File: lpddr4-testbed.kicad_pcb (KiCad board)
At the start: 6 copper layers, 69.6 x 30 mm, 68 parts, among them IC1 PCA6408APW, IC2 AT24CS01, J1 ddr4-sodimm-edge-connector, U1 MT53E1G32D2NP-046, U2 TPS613221ADBVT

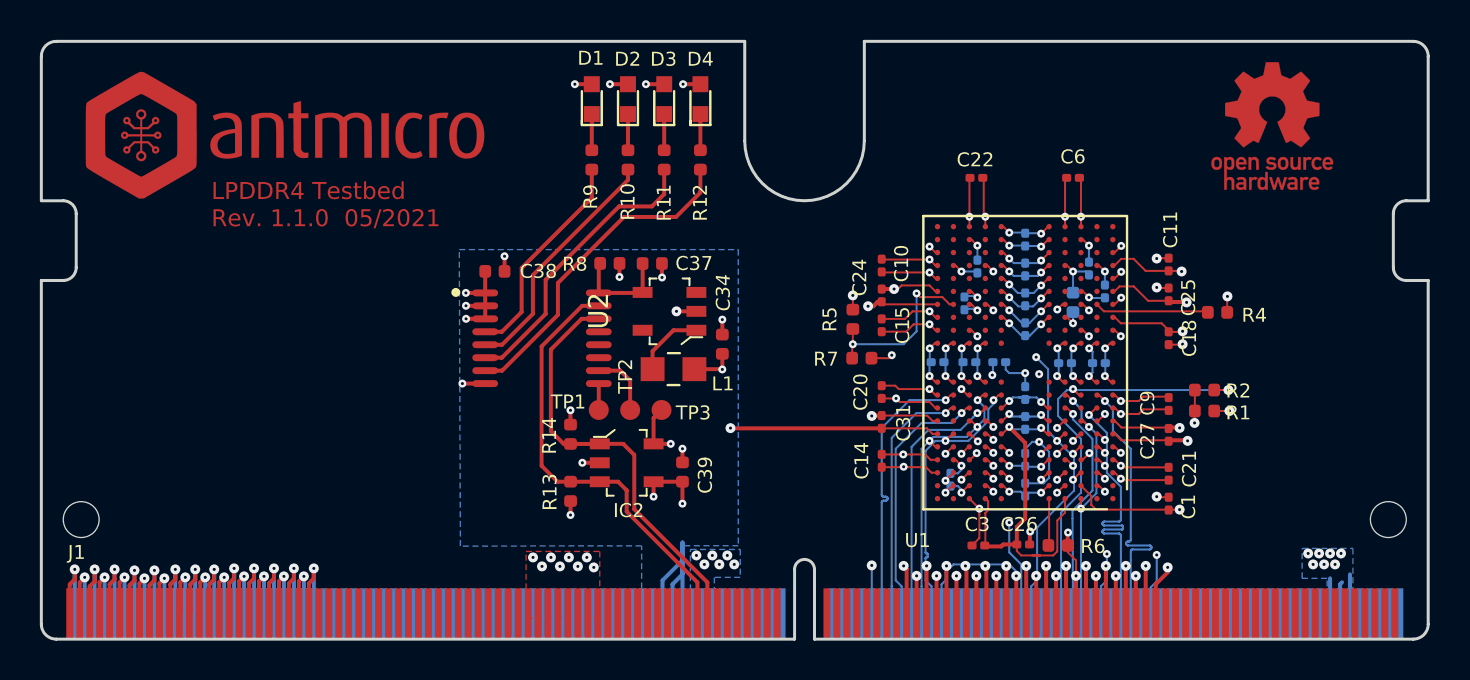
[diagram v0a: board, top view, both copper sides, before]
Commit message: Clean DRC
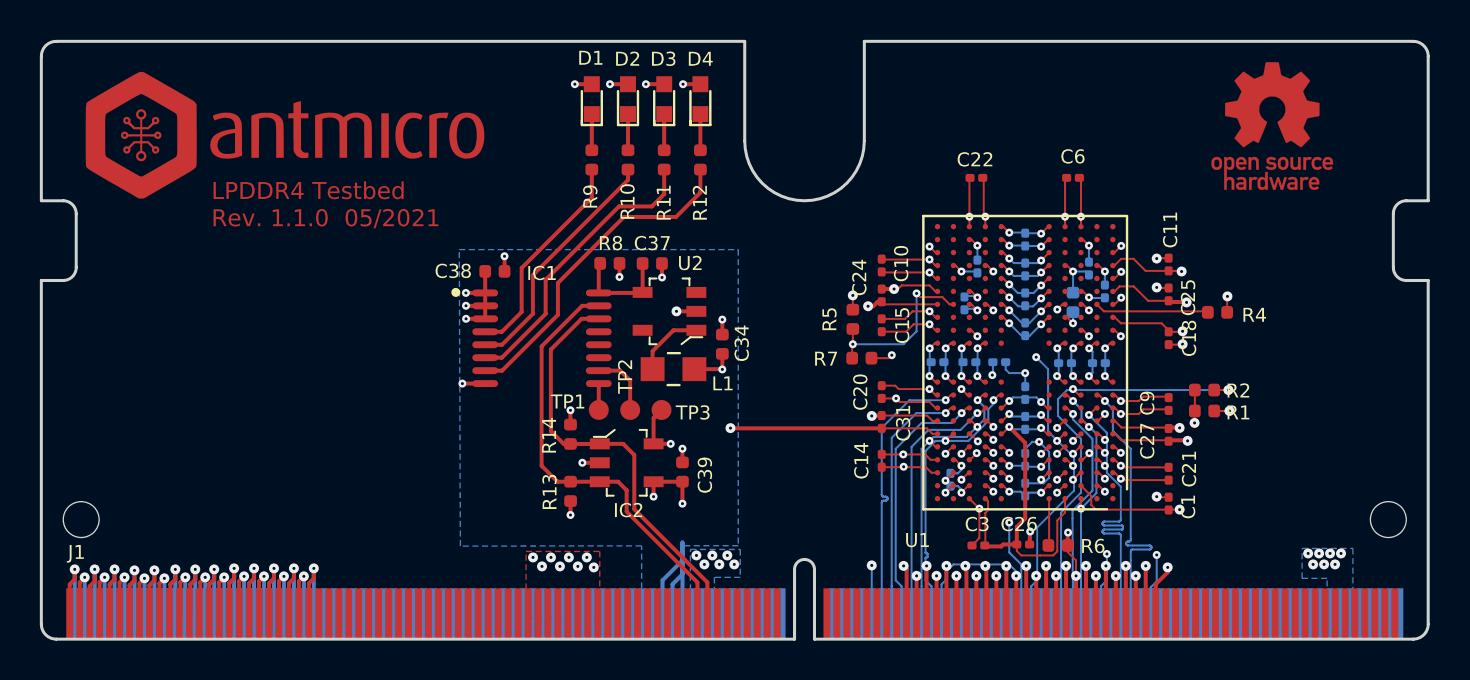
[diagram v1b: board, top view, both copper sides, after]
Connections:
- IC1 pad 11: Net-(IC1-Pad11) -> unconnected-(IC1-Pad11)
- IC1 pad 12: Net-(IC1-Pad12) -> unconnected-(IC1-Pad12)
- IC1 pad 13: Net-(IC1-Pad13) -> unconnected-(IC1-Pad13)
- J1 pad 100: Net-(J1-Pad100) -> unconnected-(J1-Pad100)
- J1 pad 102: Net-(J1-Pad102) -> unconnected-(J1-Pad102)
- J1 pad 104: Net-(J1-Pad104) -> unconnected-(J1-Pad104)
- J1 pad 106: Net-(J1-Pad106) -> unconnected-(J1-Pad106)
- J1 pad 108: Net-(J1-Pad108) -> unconnected-(J1-Pad108)
- J1 pad 109: Net-(J1-Pad109) -> unconnected-(J1-Pad109)
- J1 pad 110: Net-(J1-Pad110) -> unconnected-(J1-Pad110)
- J1 pad 111: Net-(J1-Pad111) -> unconnected-(J1-Pad111)
- J1 pad 112: Net-(J1-Pad112) -> unconnected-(J1-Pad112)
- J1 pad 113: Net-(J1-Pad113) -> unconnected-(J1-Pad113)
- J1 pad 114: Net-(J1-Pad114) -> unconnected-(J1-Pad114)
- J1 pad 115: Net-(J1-Pad115) -> unconnected-(J1-Pad115)
- J1 pad 117: Net-(J1-Pad117) -> unconnected-(J1-Pad117)
- J1 pad 119: Net-(J1-Pad119) -> unconnected-(J1-Pad119)
- J1 pad 121: Net-(J1-Pad121) -> unconnected-(J1-Pad121)
- J1 pad 123: Net-(J1-Pad123) -> unconnected-(J1-Pad123)
- J1 pad 125: Net-(J1-Pad125) -> unconnected-(J1-Pad125)
- J1 pad 131: Net-(J1-Pad131) -> unconnected-(J1-Pad131)
- J1 pad 132: Net-(J1-Pad132) -> unconnected-(J1-Pad132)
- J1 pad 133: Net-(J1-Pad133) -> unconnected-(J1-Pad133)
- J1 pad 134: Net-(J1-Pad134) -> unconnected-(J1-Pad134)
- J1 pad 135: Net-(J1-Pad135) -> unconnected-(J1-Pad135)
- J1 pad 136: Net-(J1-Pad136) -> unconnected-(J1-Pad136)
- J1 pad 137: Net-(J1-Pad137) -> unconnected-(J1-Pad137)
- J1 pad 138: Net-(J1-Pad138) -> unconnected-(J1-Pad138)
- J1 pad 139: Net-(J1-Pad139) -> unconnected-(J1-Pad139)
- J1 pad 140: Net-(J1-Pad140) -> unconnected-(J1-Pad140)
- J1 pad 141: Net-(J1-Pad141) -> unconnected-(J1-Pad141)
- J1 pad 142: Net-(J1-Pad142) -> unconnected-(J1-Pad142)
- J1 pad 143: Net-(J1-Pad143) -> unconnected-(J1-Pad143)
- J1 pad 144: Net-(J1-Pad144) -> unconnected-(J1-Pad144)
- J1 pad 145: Net-(J1-Pad145) -> unconnected-(J1-Pad145)
- J1 pad 146: Net-(J1-Pad146) -> unconnected-(J1-Pad146)
- J1 pad 147: Net-(J1-Pad147) -> unconnected-(J1-Pad147)
- J1 pad 148: Net-(J1-Pad148) -> unconnected-(J1-Pad148)
- J1 pad 149: Net-(J1-Pad149) -> unconnected-(J1-Pad149)
- J1 pad 150: Net-(J1-Pad150) -> unconnected-(J1-Pad150)
- J1 pad 151: Net-(J1-Pad151) -> unconnected-(J1-Pad151)
- J1 pad 152: Net-(J1-Pad152) -> unconnected-(J1-Pad152)
- J1 pad 153: Net-(J1-Pad153) -> unconnected-(J1-Pad153)
- J1 pad 155: Net-(J1-Pad155) -> unconnected-(J1-Pad155)
- J1 pad 157: Net-(J1-Pad157) -> unconnected-(J1-Pad157)
- J1 pad 159: Net-(J1-Pad159) -> unconnected-(J1-Pad159)
- J1 pad 170: Net-(J1-Pad170) -> unconnected-(J1-Pad170)
- J1 pad 172: Net-(J1-Pad172) -> unconnected-(J1-Pad172)
- J1 pad 174: Net-(J1-Pad174) -> unconnected-(J1-Pad174)
- J1 pad 176: Net-(J1-Pad176) -> unconnected-(J1-Pad176)
- J1 pad 178: Net-(J1-Pad178) -> unconnected-(J1-Pad178)
- J1 pad 180: Net-(J1-Pad180) -> unconnected-(J1-Pad180)
- J1 pad 182: Net-(J1-Pad182) -> unconnected-(J1-Pad182)
- J1 pad 188: Net-(J1-Pad188) -> unconnected-(J1-Pad188)
- J1 pad 190: Net-(J1-Pad190) -> unconnected-(J1-Pad190)
- J1 pad 198: Net-(J1-Pad198) -> unconnected-(J1-Pad198)
- J1 pad 202: Net-(J1-Pad202) -> unconnected-(J1-Pad202)
- J1 pad 208: Net-(J1-Pad208) -> unconnected-(J1-Pad208)
- J1 pad 212: Net-(J1-Pad212) -> unconnected-(J1-Pad212)
- J1 pad 213: Net-(J1-Pad213) -> unconnected-(J1-Pad213)
- J1 pad 214: Net-(J1-Pad214) -> unconnected-(J1-Pad214)
- J1 pad 215: Net-(J1-Pad215) -> unconnected-(J1-Pad215)
- J1 pad 216: Net-(J1-Pad216) -> unconnected-(J1-Pad216)
- J1 pad 217: Net-(J1-Pad217) -> unconnected-(J1-Pad217)
- J1 pad 218: Net-(J1-Pad218) -> unconnected-(J1-Pad218)
- J1 pad 219: Net-(J1-Pad219) -> unconnected-(J1-Pad219)
- J1 pad 220: Net-(J1-Pad220) -> unconnected-(J1-Pad220)
- J1 pad 221: Net-(J1-Pad221) -> unconnected-(J1-Pad221)
- J1 pad 222: Net-(J1-Pad222) -> unconnected-(J1-Pad222)
- J1 pad 223: Net-(J1-Pad223) -> unconnected-(J1-Pad223)
- J1 pad 224: Net-(J1-Pad224) -> unconnected-(J1-Pad224)
- J1 pad 225: Net-(J1-Pad225) -> unconnected-(J1-Pad225)
- J1 pad 226: Net-(J1-Pad226) -> unconnected-(J1-Pad226)
- J1 pad 227: Net-(J1-Pad227) -> unconnected-(J1-Pad227)
- J1 pad 228: Net-(J1-Pad228) -> unconnected-(J1-Pad228)
- J1 pad 229: Net-(J1-Pad229) -> unconnected-(J1-Pad229)
- J1 pad 230: Net-(J1-Pad230) -> unconnected-(J1-Pad230)
- J1 pad 231: Net-(J1-Pad231) -> unconnected-(J1-Pad231)
- J1 pad 232: Net-(J1-Pad232) -> unconnected-(J1-Pad232)
- J1 pad 233: Net-(J1-Pad233) -> unconnected-(J1-Pad233)
- J1 pad 234: Net-(J1-Pad234) -> unconnected-(J1-Pad234)
- J1 pad 235: Net-(J1-Pad235) -> unconnected-(J1-Pad235)
- J1 pad 236: Net-(J1-Pad236) -> unconnected-(J1-Pad236)
- J1 pad 237: Net-(J1-Pad237) -> unconnected-(J1-Pad237)
- J1 pad 238: Net-(J1-Pad238) -> unconnected-(J1-Pad238)
- J1 pad 239: Net-(J1-Pad239) -> unconnected-(J1-Pad239)
- J1 pad 240: Net-(J1-Pad240) -> unconnected-(J1-Pad240)
- J1 pad 241: Net-(J1-Pad241) -> unconnected-(J1-Pad241)
- J1 pad 242: Net-(J1-Pad242) -> unconnected-(J1-Pad242)
- J1 pad 243: Net-(J1-Pad243) -> unconnected-(J1-Pad243)
- J1 pad 244: Net-(J1-Pad244) -> unconnected-(J1-Pad244)
- J1 pad 245: Net-(J1-Pad245) -> unconnected-(J1-Pad245)
- J1 pad 247: Net-(J1-Pad247) -> unconnected-(J1-Pad247)
- J1 pad 249: Net-(J1-Pad249) -> unconnected-(J1-Pad249)
- J1 pad 251: Net-(J1-Pad251) -> unconnected-(J1-Pad251)
- J1 pad 252: Net-(J1-Pad252) -> unconnected-(J1-Pad252)
- J1 pad 253: Net-(J1-Pad253) -> unconnected-(J1-Pad253)
- J1 pad 254: Net-(J1-Pad254) -> unconnected-(J1-Pad254)
- J1 pad 255: Net-(J1-Pad255) -> unconnected-(J1-Pad255)
- J1 pad 256: Net-(J1-Pad256) -> unconnected-(J1-Pad256)
- J1 pad 257: Net-(J1-Pad257) -> unconnected-(J1-Pad257)
- J1 pad 258: Net-(J1-Pad258) -> unconnected-(J1-Pad258)
- J1 pad 259: Net-(J1-Pad259) -> unconnected-(J1-Pad259)
- J1 pad 260: Net-(J1-Pad260) -> unconnected-(J1-Pad260)
- J1 pad 51: Net-(J1-Pad51) -> unconnected-(J1-Pad51)
- J1 pad 52: Net-(J1-Pad52) -> unconnected-(J1-Pad52)
- J1 pad 53: Net-(J1-Pad53) -> unconnected-(J1-Pad53)
- J1 pad 54: Net-(J1-Pad54) -> unconnected-(J1-Pad54)
- J1 pad 55: Net-(J1-Pad55) -> unconnected-(J1-Pad55)
- J1 pad 56: Net-(J1-Pad56) -> unconnected-(J1-Pad56)
- J1 pad 57: Net-(J1-Pad57) -> unconnected-(J1-Pad57)
- J1 pad 58: Net-(J1-Pad58) -> unconnected-(J1-Pad58)
- J1 pad 59: Net-(J1-Pad59) -> unconnected-(J1-Pad59)
- J1 pad 60: Net-(J1-Pad60) -> unconnected-(J1-Pad60)
- J1 pad 61: Net-(J1-Pad61) -> unconnected-(J1-Pad61)
- J1 pad 62: Net-(J1-Pad62) -> unconnected-(J1-Pad62)
- J1 pad 63: Net-(J1-Pad63) -> unconnected-(J1-Pad63)
- J1 pad 64: Net-(J1-Pad64) -> unconnected-(J1-Pad64)
- J1 pad 65: Net-(J1-Pad65) -> unconnected-(J1-Pad65)
- J1 pad 66: Net-(J1-Pad66) -> unconnected-(J1-Pad66)
- J1 pad 67: Net-(J1-Pad67) -> unconnected-(J1-Pad67)
- J1 pad 68: Net-(J1-Pad68) -> unconnected-(J1-Pad68)
- J1 pad 69: Net-(J1-Pad69) -> unconnected-(J1-Pad69)
- J1 pad 70: Net-(J1-Pad70) -> unconnected-(J1-Pad70)
- J1 pad 71: Net-(J1-Pad71) -> unconnected-(J1-Pad71)
- J1 pad 72: Net-(J1-Pad72) -> unconnected-(J1-Pad72)
- J1 pad 73: Net-(J1-Pad73) -> unconnected-(J1-Pad73)
- J1 pad 74: Net-(J1-Pad74) -> unconnected-(J1-Pad74)
- J1 pad 75: Net-(J1-Pad75) -> unconnected-(J1-Pad75)
- J1 pad 76: Net-(J1-Pad76) -> unconnected-(J1-Pad76)
- J1 pad 77: Net-(J1-Pad77) -> unconnected-(J1-Pad77)
- J1 pad 78: Net-(J1-Pad78) -> unconnected-(J1-Pad78)
- J1 pad 79: Net-(J1-Pad79) -> unconnected-(J1-Pad79)
- J1 pad 80: Net-(J1-Pad80) -> unconnected-(J1-Pad80)
- J1 pad 81: Net-(J1-Pad81) -> unconnected-(J1-Pad81)
- J1 pad 82: Net-(J1-Pad82) -> unconnected-(J1-Pad82)
- J1 pad 83: Net-(J1-Pad83) -> unconnected-(J1-Pad83)
- J1 pad 84: Net-(J1-Pad84) -> unconnected-(J1-Pad84)
- J1 pad 85: Net-(J1-Pad85) -> unconnected-(J1-Pad85)
- J1 pad 86: Net-(J1-Pad86) -> unconnected-(J1-Pad86)
- J1 pad 87: Net-(J1-Pad87) -> unconnected-(J1-Pad87)
- J1 pad 88: Net-(J1-Pad88) -> unconnected-(J1-Pad88)
- J1 pad 89: Net-(J1-Pad89) -> unconnected-(J1-Pad89)
- J1 pad 90: Net-(J1-Pad90) -> unconnected-(J1-Pad90)
- J1 pad 91: Net-(J1-Pad91) -> unconnected-(J1-Pad91)
- J1 pad 92: Net-(J1-Pad92) -> unconnected-(J1-Pad92)
- J1 pad 94: Net-(J1-Pad94) -> unconnected-(J1-Pad94)
- J1 pad 96: Net-(J1-Pad96) -> unconnected-(J1-Pad96)
- J1 pad 98: Net-(J1-Pad98) -> unconnected-(J1-Pad98)
- U1 pad A1: Net-(U1-PadA1) -> unconnected-(U1-PadA1)
- U1 pad A11: Net-(U1-PadA11) -> unconnected-(U1-PadA11)
- U1 pad A12: Net-(U1-PadA12) -> unconnected-(U1-PadA12)
- U1 pad A2: Net-(U1-PadA2) -> unconnected-(U1-PadA2)
- U1 pad A8: Net-(U1-PadA8) -> unconnected-(U1-PadA8)
- U1 pad AA1: Net-(U1-PadAA1) -> unconnected-(U1-PadAA1)
- U1 pad AA11: Net-(U1-PadAA11) -> unconnected-(U1-PadAA11)
- U1 pad AA12: Net-(U1-PadAA12) -> unconnected-(U1-PadAA12)
- U1 pad AA2: Net-(U1-PadAA2) -> unconnected-(U1-PadAA2)
- U1 pad AA4: Net-(U1-PadAA4) -> unconnected-(U1-PadAA4)
- U1 pad AA9: Net-(U1-PadAA9) -> unconnected-(U1-PadAA9)
- U1 pad AB1: Net-(U1-PadAB1) -> unconnected-(U1-PadAB1)
- U1 pad AB11: Net-(U1-PadAB11) -> unconnected-(U1-PadAB11)
- U1 pad AB12: Net-(U1-PadAB12) -> unconnected-(U1-PadAB12)
- U1 pad AB2: Net-(U1-PadAB2) -> unconnected-(U1-PadAB2)
- U1 pad B1: Net-(U1-PadB1) -> unconnected-(U1-PadB1)
- U1 pad B12: Net-(U1-PadB12) -> unconnected-(U1-PadB12)
- U1 pad G11: Net-(U1-PadG11) -> unconnected-(U1-PadG11)
- U1 pad H3: Net-(U1-PadH3) -> unconnected-(U1-PadH3)
- U1 pad J5: Net-(U1-PadJ5) -> unconnected-(U1-PadJ5)
- U1 pad K5: Net-(U1-PadK5) -> unconnected-(U1-PadK5)
- U1 pad K8: Net-(U1-PadK8) -> unconnected-(U1-PadK8)
- U1 pad N5: Net-(U1-PadN5) -> unconnected-(U1-PadN5)
- U1 pad N8: Net-(U1-PadN8) -> unconnected-(U1-PadN8)
- U1 pad P11: Net-(U1-PadP11) -> unconnected-(U1-PadP11)
- U1 pad P2: Net-(U1-PadP2) -> unconnected-(U1-PadP2)
- U1 pad P4: Net-(U1-PadP4) -> unconnected-(U1-PadP4)
- U1 pad P5: Net-(U1-PadP5) -> unconnected-(U1-PadP5)
- U1 pad P8: Net-(U1-PadP8) -> unconnected-(U1-PadP8)
- U1 pad P9: Net-(U1-PadP9) -> unconnected-(U1-PadP9)
- U1 pad R10: Net-(U1-PadR10) -> unconnected-(U1-PadR10)
- U1 pad R11: Net-(U1-PadR11) -> unconnected-(U1-PadR11)
- U1 pad R2: Net-(U1-PadR2) -> unconnected-(U1-PadR2)
- U1 pad R3: Net-(U1-PadR3) -> unconnected-(U1-PadR3)
- U1 pad R9: Net-(U1-PadR9) -> unconnected-(U1-PadR9)
- U1 pad U11: Net-(U1-PadU11) -> unconnected-(U1-PadU11)
- U1 pad U2: Net-(U1-PadU2) -> unconnected-(U1-PadU2)
- U1 pad U4: Net-(U1-PadU4) -> unconnected-(U1-PadU4)
- U1 pad U9: Net-(U1-PadU9) -> unconnected-(U1-PadU9)
- U1 pad V10: Net-(U1-PadV10) -> unconnected-(U1-PadV10)
- U1 pad V11: Net-(U1-PadV11) -> unconnected-(U1-PadV11)
- U1 pad V2: Net-(U1-PadV2) -> unconnected-(U1-PadV2)
- U1 pad V3: Net-(U1-PadV3) -> unconnected-(U1-PadV3)
- U1 pad V4: Net-(U1-PadV4) -> unconnected-(U1-PadV4)
- U1 pad V9: Net-(U1-PadV9) -> unconnected-(U1-PadV9)
- U1 pad W10: Net-(U1-PadW10) -> unconnected-(U1-PadW10)
- U1 pad W3: Net-(U1-PadW3) -> unconnected-(U1-PadW3)
- U1 pad Y10: Net-(U1-PadY10) -> unconnected-(U1-PadY10)
- U1 pad Y11: Net-(U1-PadY11) -> unconnected-(U1-PadY11)
- U1 pad Y2: Net-(U1-PadY2) -> unconnected-(U1-PadY2)
- U1 pad Y3: Net-(U1-PadY3) -> unconnected-(U1-PadY3)
- U1 pad Y4: Net-(U1-PadY4) -> unconnected-(U1-PadY4)
- U1 pad Y9: Net-(U1-PadY9) -> unconnected-(U1-PadY9)
- U2 pad 3: Net-(U2-Pad3) -> unconnected-(U2-Pad3)
- U2 pad 5: Net-(U2-Pad5) -> unconnected-(U2-Pad5)
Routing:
- net VDDQ: track 44.7 -> 39.1 mm
- net VDD2: track 57.0 -> 55.6 mm
- net GND: track 237.4 -> 236.3 mm
- net VDD1: track 100.3 -> 100.2 mm, vias 19 -> 18
